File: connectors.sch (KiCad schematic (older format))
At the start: 36 parts, among them J10 UART_R1, J4 Conn_01x04_Male, J8 Conn_01x05, J9 UART_L1

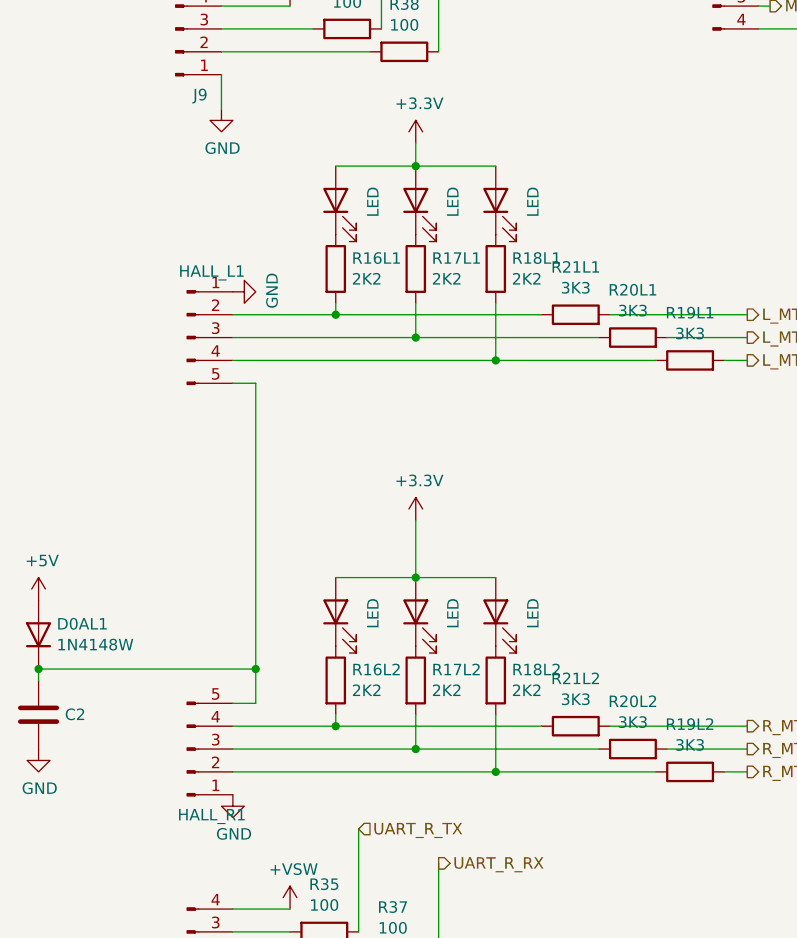
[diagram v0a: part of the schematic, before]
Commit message: finish design
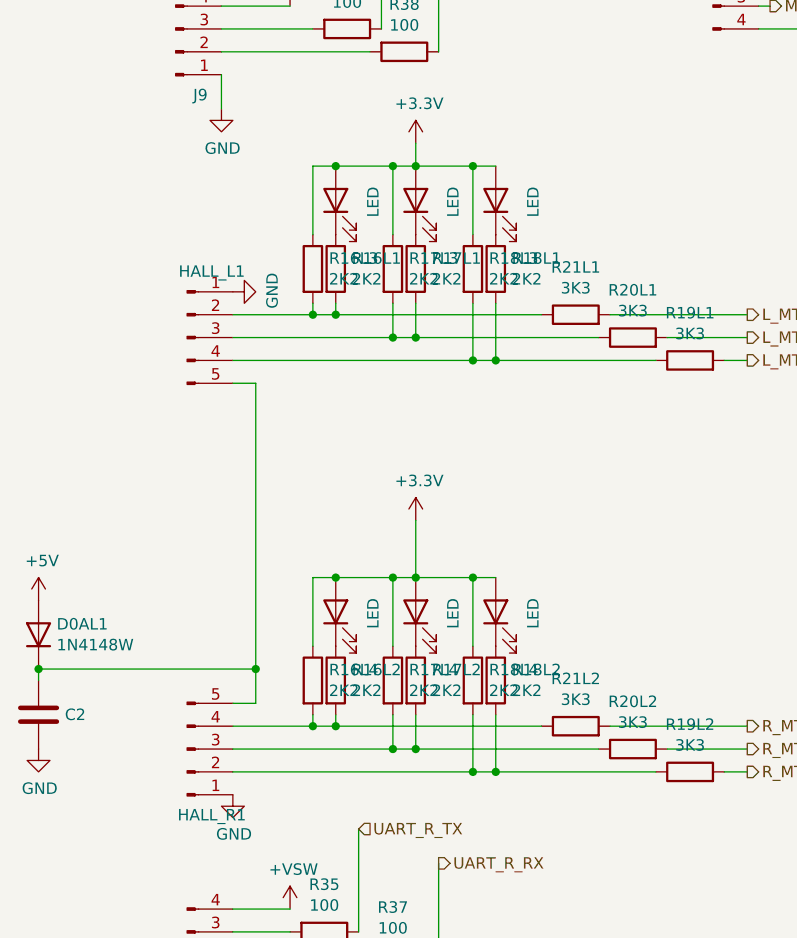
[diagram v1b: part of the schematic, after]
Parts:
- added R16L3, R16L4, R17L3, R17L4, R18L3, R18L4: 2K2, Resistor_SMD:R_0603_1608Metric, symbol Device:R
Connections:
- net +3V3: now also R16L3.1, R16L4.1, R17L3.1, R17L4.1, R18L3.1, R18L4.1
- net at HALL_L1.2 (Pin_2), R16L1.2, R21L1.1: now also R16L3.2
- net at HALL_L1.3 (Pin_3), R17L1.2, R20L1.1: now also R17L3.2
- net at HALL_L1.4 (Pin_4), R18L1.2, R19L1.1: now also R18L3.2
- net at HALL_R1.2 (Pin_2), R18L2.2, R19L2.1: now also R18L4.2
- net at HALL_R1.3 (Pin_3), R17L2.2, R20L2.1: now also R17L4.2
- net at HALL_R1.4 (Pin_4), R16L2.2, R21L2.1: now also R16L4.2
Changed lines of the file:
@@
 $EndComp
-Wire Wire Line
-	2450 2600 2900 2600
 Wire Wire Line
 	4050 2700 3250 2700
 Wire Wire Line
-	2450 2800 3600 2800
+	2450 2800 3500 2800
 Wire Wire Line
 	2900 2550 2900 2600
 Connection ~ 2900 2600
 Wire Wire Line
-	2900 2600 3800 2600
-Wire Wire Line
 	3250 2550 3250 2700
 Connection ~ 3250 2700
-Wire Wire Line
-	3250 2700 2450 2700
 Wire Wire Line
 	3600 2550 3600 2800
@@
 $EndComp
 Wire Wire Line
-	2450 4400 2900 4400
+	2450 4400 2800 4400
 Wire Wire Line
 	4050 4500 3250 4500
-Wire Wire Line
-	2450 4600 3600 4600
 Wire Wire Line
 	2900 4350 2900 4400
 Connection ~ 2900 4400
 Wire Wire Line
-	2900 4400 3800 4400
-Wire Wire Line
 	3250 4350 3250 4500
 Connection ~ 3250 4500
 Wire Wire Line
-	3250 4500 2450 4500
+	3250 4500 3150 4500
 Wire Wire Line
 	3600 4350 3600 4600
@@
 $EndComp
 Wire Wire Line
-	2900 1950 3250 1950
+	2900 1950 3150 1950
 Connection ~ 3250 1950
 Wire Wire Line
-	3250 1950 3600 1950
+	3250 1950 3500 1950
 Wire Wire Line
 	3250 1850 3250 1950
@@
 $EndComp
 Wire Wire Line
-	2900 3750 3250 3750
+	2900 3750 3150 3750
 Connection ~ 3250 3750
 Wire Wire Line
-	3250 3750 3600 3750
+	3250 3750 3500 3750
 Wire Wire Line
 	3250 3500 3250 3750
+$Comp
+L Device:R R16L3
+U 1 1 5F8901AA
+P 2800 2400
+F 0 "R16L3" H 2870 2446 50  0000 L CNN
+F 1 "2K2" H 2870 2355 50  0000 L CNN
+F 2 "Resistor_SMD:R_0603_1608Metric" V 2730 2400 50  0001 C CNN
+F 3 "~" H 2800 2400 50  0001 C CNN
+	1    2800 2400
+	1    0    0    -1
+$EndComp
+$Comp
+L Device:R R17L3
+U 1 1 5F890945
+P 3150 2400
+F 0 "R17L3" H 3220 2446 50  0000 L CNN
+F 1 "2K2" H 3220 2355 50  0000 L CNN
+F 2 "Resistor_SMD:R_0603_1608Metric" V 3080 2400 50  0001 C CNN
+F 3 "~" H 3150 2400 50  0001 C CNN
+	1    3150 2400
+	1    0    0    -1
+$EndComp
+$Comp
+L Device:R R18L3
+U 1 1 5F890B23
+P 3500 2400
+F 0 "R18L3" H 3570 2446 50  0000 L CNN
+F 1 "2K2" H 3570 2355 50  0000 L CNN
+F 2 "Resistor_SMD:R_0603_1608Metric" V 3430 2400 50  0001 C CNN
+F 3 "~" H 3500 2400 50  0001 C CNN
+	1    3500 2400
+	1    0    0    -1
+$EndComp
+Wire Wire Line
+	2450 2600 2800 2600
+Wire Wire Line
+	2800 2550 2800 2600
+Connection ~ 2800 2600
+Wire Wire Line
+	2800 2600 2900 2600
+Wire Wire Line
+	3500 2250 3500 1950
+Connection ~ 3500 1950
+Wire Wire Line
+	3500 1950 3600 1950
+Wire Wire Line
+	3150 2250 3150 1950
+Connection ~ 3150 1950
+Wire Wire Line
+	3150 1950 3250 1950
+Wire Wire Line
+	2800 2250 2800 1950
+Wire Wire Line
+	2800 1950 2900 1950
+Connection ~ 2900 1950
+$Comp
+L Device:R R16L4
+U 1 1 5F8A0AE7
+P 2800 4200
+F 0 "R16L4" H 2870 4246 50  0000 L CNN
+F 1 "2K2" H 2870 4155 50  0000 L CNN
+F 2 "Resistor_SMD:R_0603_1608Metric" V 2730 4200 50  0001 C CNN
+F 3 "~" H 2800 4200 50  0001 C CNN
+	1    2800 4200
+	1    0    0    -1
+$EndComp
+$Comp
+L Device:R R17L4
+U 1 1 5F8A0C56
+P 3150 4200
+F 0 "R17L4" H 3220 4246 50  0000 L CNN
+F 1 "2K2" H 3220 4155 50  0000 L CNN
+F 2 "Resistor_SMD:R_0603_1608Metric" V 3080 4200 50  0001 C CNN
+F 3 "~" H 3150 4200 50  0001 C CNN
+	1    3150 4200
+	1    0    0    -1
+$EndComp
+$Comp
+L Device:R R18L4
+U 1 1 5F8A0DC6
+P 3500 4200
+F 0 "R18L4" H 3570 4246 50  0000 L CNN
+F 1 "2K2" H 3570 4155 50  0000 L CNN
+F 2 "Resistor_SMD:R_0603_1608Metric" V 3430 4200 50  0001 C CNN
+F 3 "~" H 3500 4200 50  0001 C CNN
+	1    3500 4200
+	1    0    0    -1
+$EndComp
+Wire Wire Line
+	2800 4350 2800 4400
+Connection ~ 2800 4400
+Wire Wire Line
+	2800 4400 2900 4400
+Wire Wire Line
+	3500 4050 3500 3750
+Connection ~ 3500 3750
+Wire Wire Line
+	3500 3750 3600 3750
+Wire Wire Line
+	3150 4050 3150 3750
+Connection ~ 3150 3750
+Wire Wire Line
+	3150 3750 3250 3750
+Wire Wire Line
+	2800 4050 2800 3750
+Wire Wire Line
+	2800 3750 2900 3750
+Connection ~ 2900 3750
+Wire Wire Line
+	2900 4400 3800 4400
+Wire Wire Line
+	2450 4600 3500 4600
+Wire Wire Line
+	3150 4350 3150 4500
+Connection ~ 3150 4500
+Wire Wire Line
+	3150 4500 2450 4500
+Wire Wire Line
+	3500 4350 3500 4600
+Connection ~ 3500 4600
+Wire Wire Line
+	3500 4600 3600 4600
+Wire Wire Line
+	3250 2700 3150 2700
+Wire Wire Line
+	2900 2600 3800 2600
+Wire Wire Line
+	3150 2550 3150 2700
+Connection ~ 3150 2700
+Wire Wire Line
+	3150 2700 2450 2700
+Wire Wire Line
+	3500 2550 3500 2800
+Connection ~ 3500 2800
+Wire Wire Line
+	3500 2800 3600 2800
 $EndSCHEMATC
